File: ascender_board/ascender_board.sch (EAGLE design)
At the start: 92 parts, among them Q1 8MHz, U1 STM32F722XX, U2 LM5107MA, U3 LM5107MA, U4 LM5107MA, U5 LM5107MA, U6 LM5107MA, U7 LM5107MA, X1 MINI-USB-32005-201

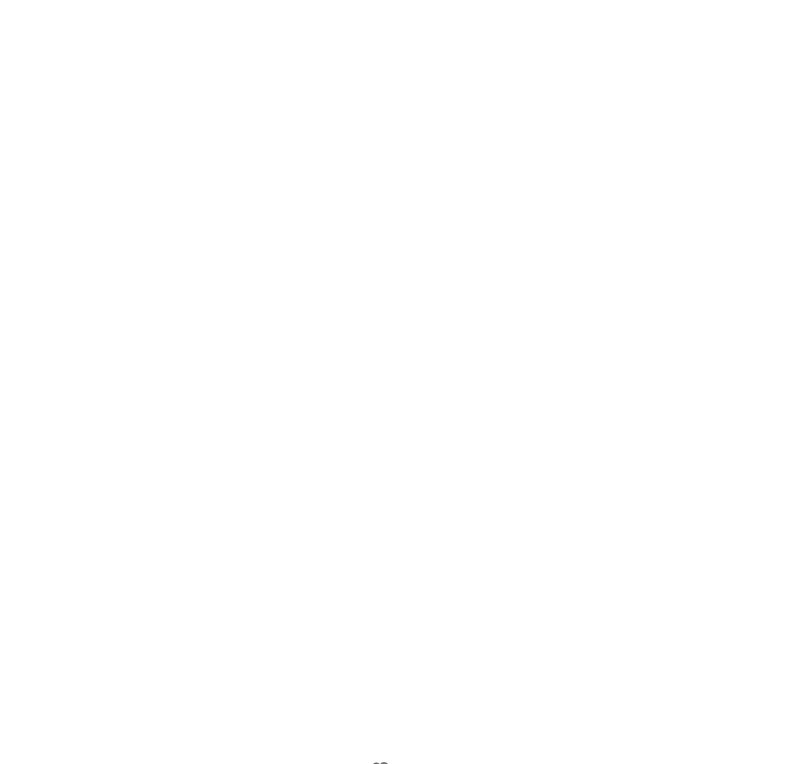
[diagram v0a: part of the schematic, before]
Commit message: board
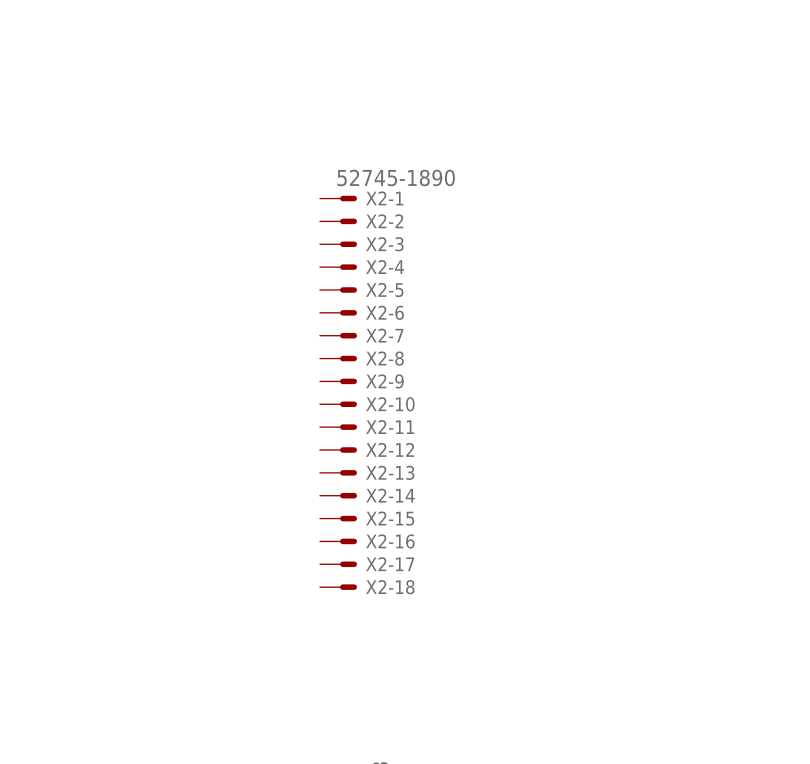
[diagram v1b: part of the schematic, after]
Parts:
- added X2: 52745-1890, con-molex:52745-1890
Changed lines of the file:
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@@
 <part name="GND54" library="supply1" deviceset="GND" device=""/>
 <part name="+3V23" library="supply1" deviceset="+3V3" device=""/>
+<part name="X2" library="con-molex" deviceset="52745-1890" device=""/>
 </parts>
 <sheets>
@@
 <instance part="GND54" gate="1" x="424.18" y="127"/>
 <instance part="+3V23" gate="G$1" x="424.18" y="175.26"/>
+<instance part="X2" gate="-1" x="365.76" y="294.64"/>
+<instance part="X2" gate="-2" x="365.76" y="292.1"/>
+<instance part="X2" gate="-3" x="365.76" y="289.56"/>
+<instance part="X2" gate="-4" x="365.76" y="287.02"/>
+<instance part="X2" gate="-5" x="365.76" y="284.48"/>
+<instance part="X2" gate="-6" x="365.76" y="281.94"/>
+<instance part="X2" gate="-7" x="365.76" y="279.4"/>
+<instance part="X2" gate="-8" x="365.76" y="276.86"/>
+<instance part="X2" gate="-9" x="365.76" y="274.32"/>
+<instance part="X2" gate="-10" x="365.76" y="271.78"/>
+<instance part="X2" gate="-11" x="365.76" y="269.24"/>
+<instance part="X2" gate="-12" x="365.76" y="266.7"/>
+<instance part="X2" gate="-13" x="365.76" y="264.16"/>
+<instance part="X2" gate="-14" x="365.76" y="261.62"/>
+<instance part="X2" gate="-15" x="365.76" y="259.08"/>
+<instance part="X2" gate="-16" x="365.76" y="256.54"/>
+<instance part="X2" gate="-17" x="365.76" y="254"/>
+<instance part="X2" gate="-18" x="365.76" y="251.46"/>
 </instances>
 <busses>

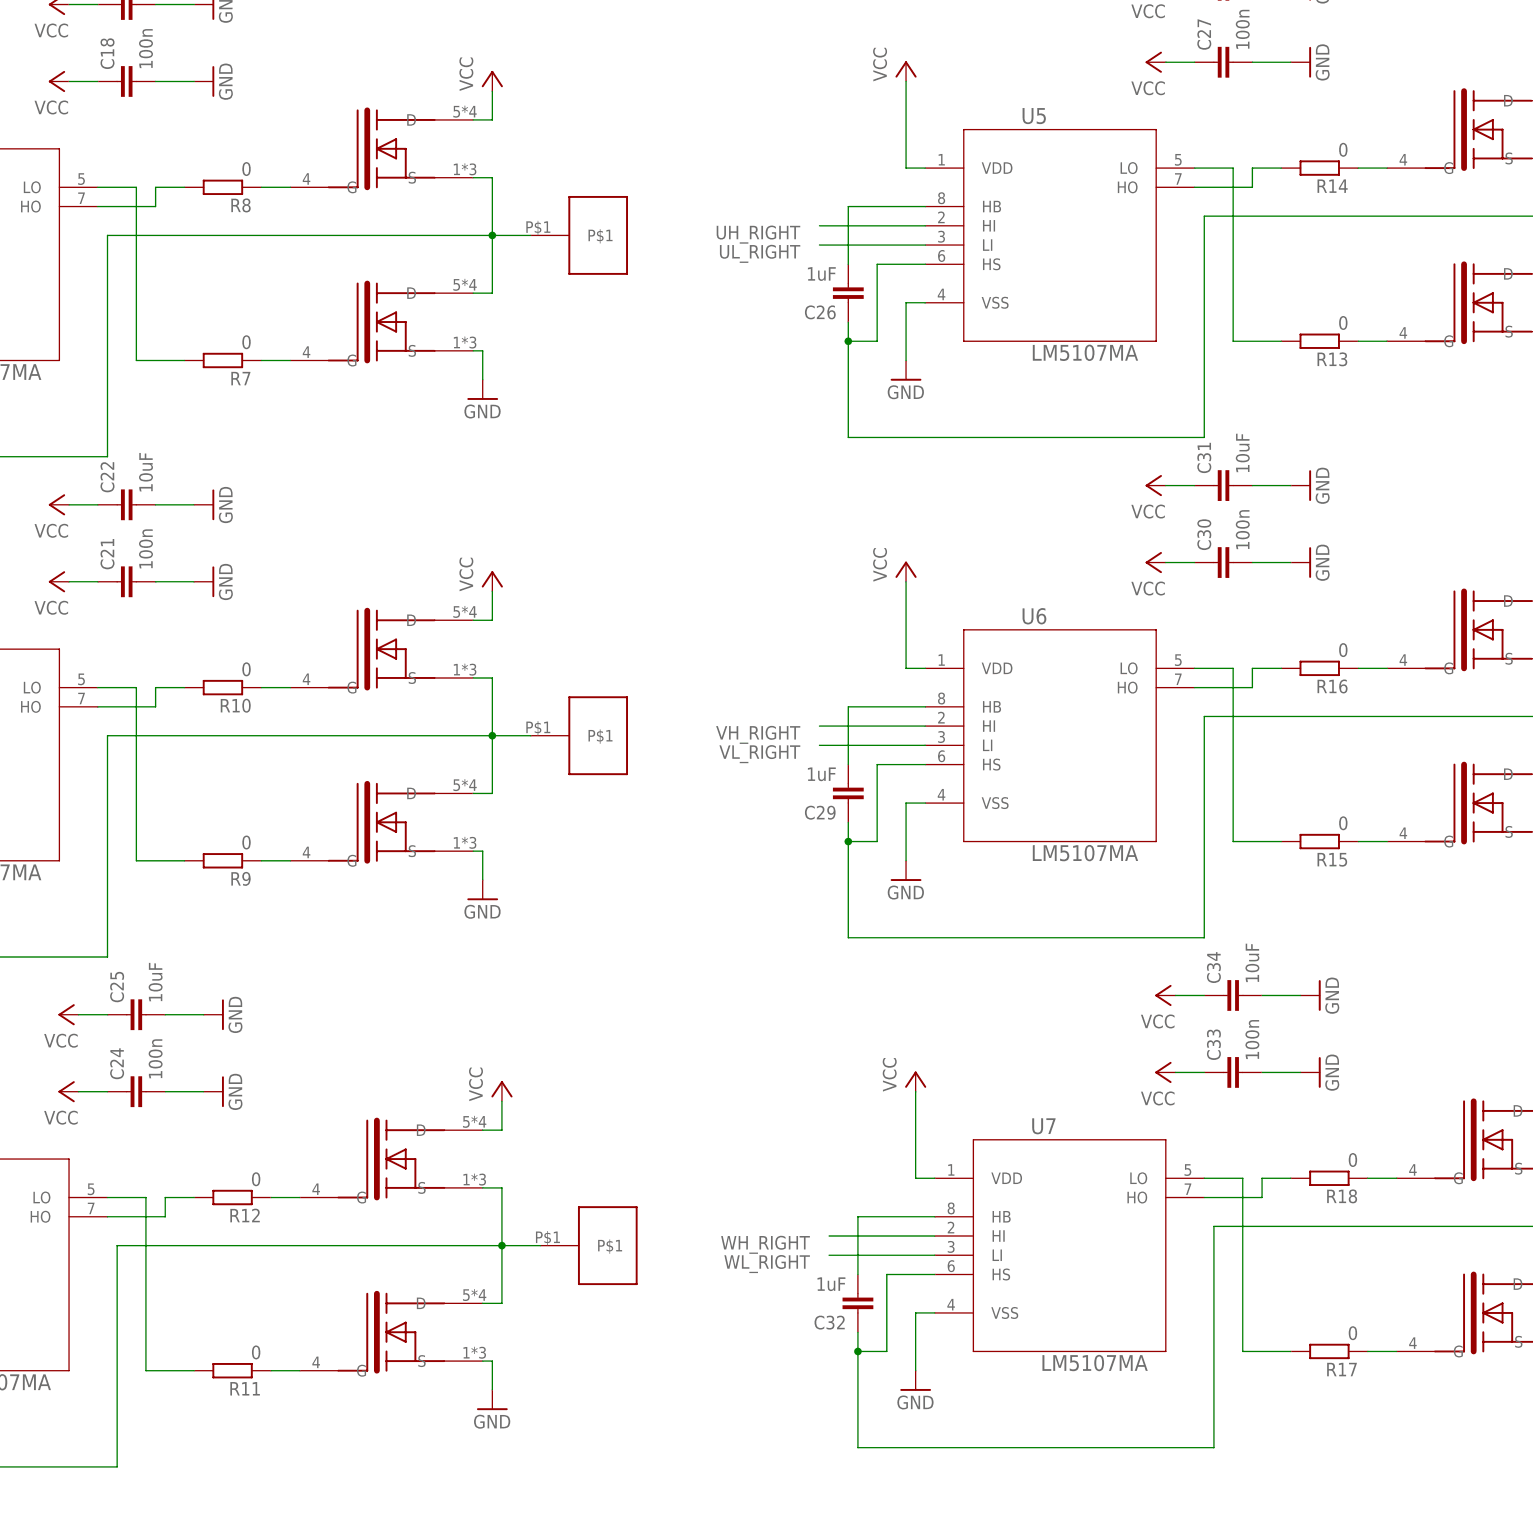
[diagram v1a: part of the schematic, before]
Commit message: board
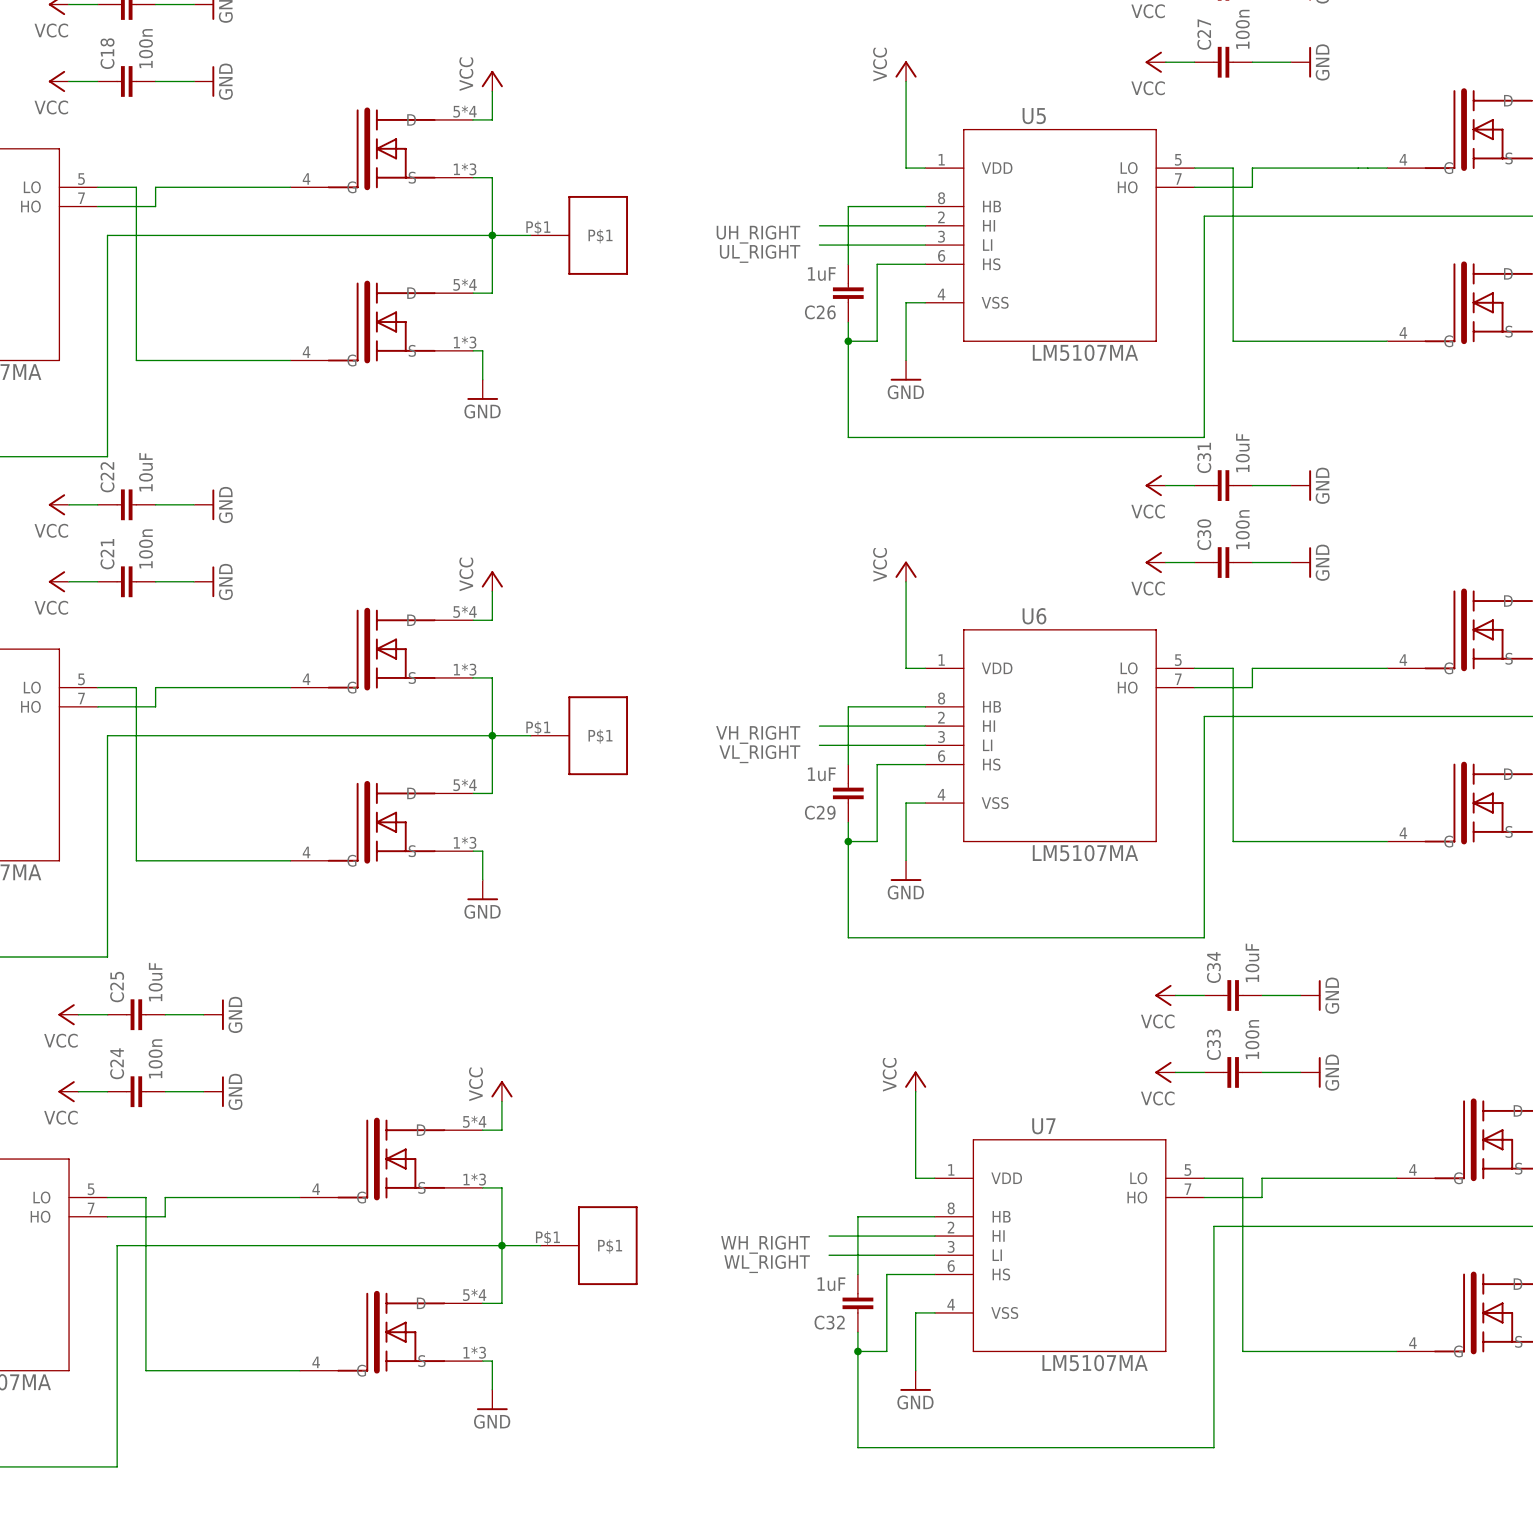
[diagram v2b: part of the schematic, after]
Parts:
- removed R10, R11, R12, R13, R14, R15, R16, R17, R18, R7, R8, R9: 0, resistor:R-EU_M0805
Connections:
- removed net N$12: R8.1, U$4.G
- removed net N$13: R9.2, U3.LO
- removed net N$17: R10.1, U$7.G
- removed net N$21: R11.2, U4.LO
- removed net N$23: R12.1, U$10.G
- removed net N$26: R13.1, U$14.G
- removed net N$29: R14.1, U$13.G
- removed net N$33: R15.2, U6.LO
- removed net N$35: R16.1, U$16.G
- removed net N$39: R17.2, U7.LO
- removed net N$41: R18.1, U$19.G
- removed net N$8: R7.1, U$5.G
- net N$10: now also U$4.G; no longer R8.2
- net N$14: now also U$7.G; no longer R10.2
- net N$20: now also U4.LO; no longer R11.1
- net N$22: now also U$10.G; no longer R12.2
- net N$27: now also U$14.G; no longer R13.2
- net N$28: now also U$13.G; no longer R14.2
- net N$32: now also U6.LO; no longer R15.1
- net N$34: now also U$16.G; no longer R16.2
- net N$38: now also U7.LO; no longer R17.1
- net N$40: now also U$19.G; no longer R18.2
- net N$7: now also U3.LO; no longer R9.1
- net N$9: now also U$5.G; no longer R7.2
